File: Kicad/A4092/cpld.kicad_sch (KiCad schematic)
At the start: 15 parts, among them J2 Conn_01x06_Pin, U7 AMS1117-3.3, U9 XC95144XL-TQ144

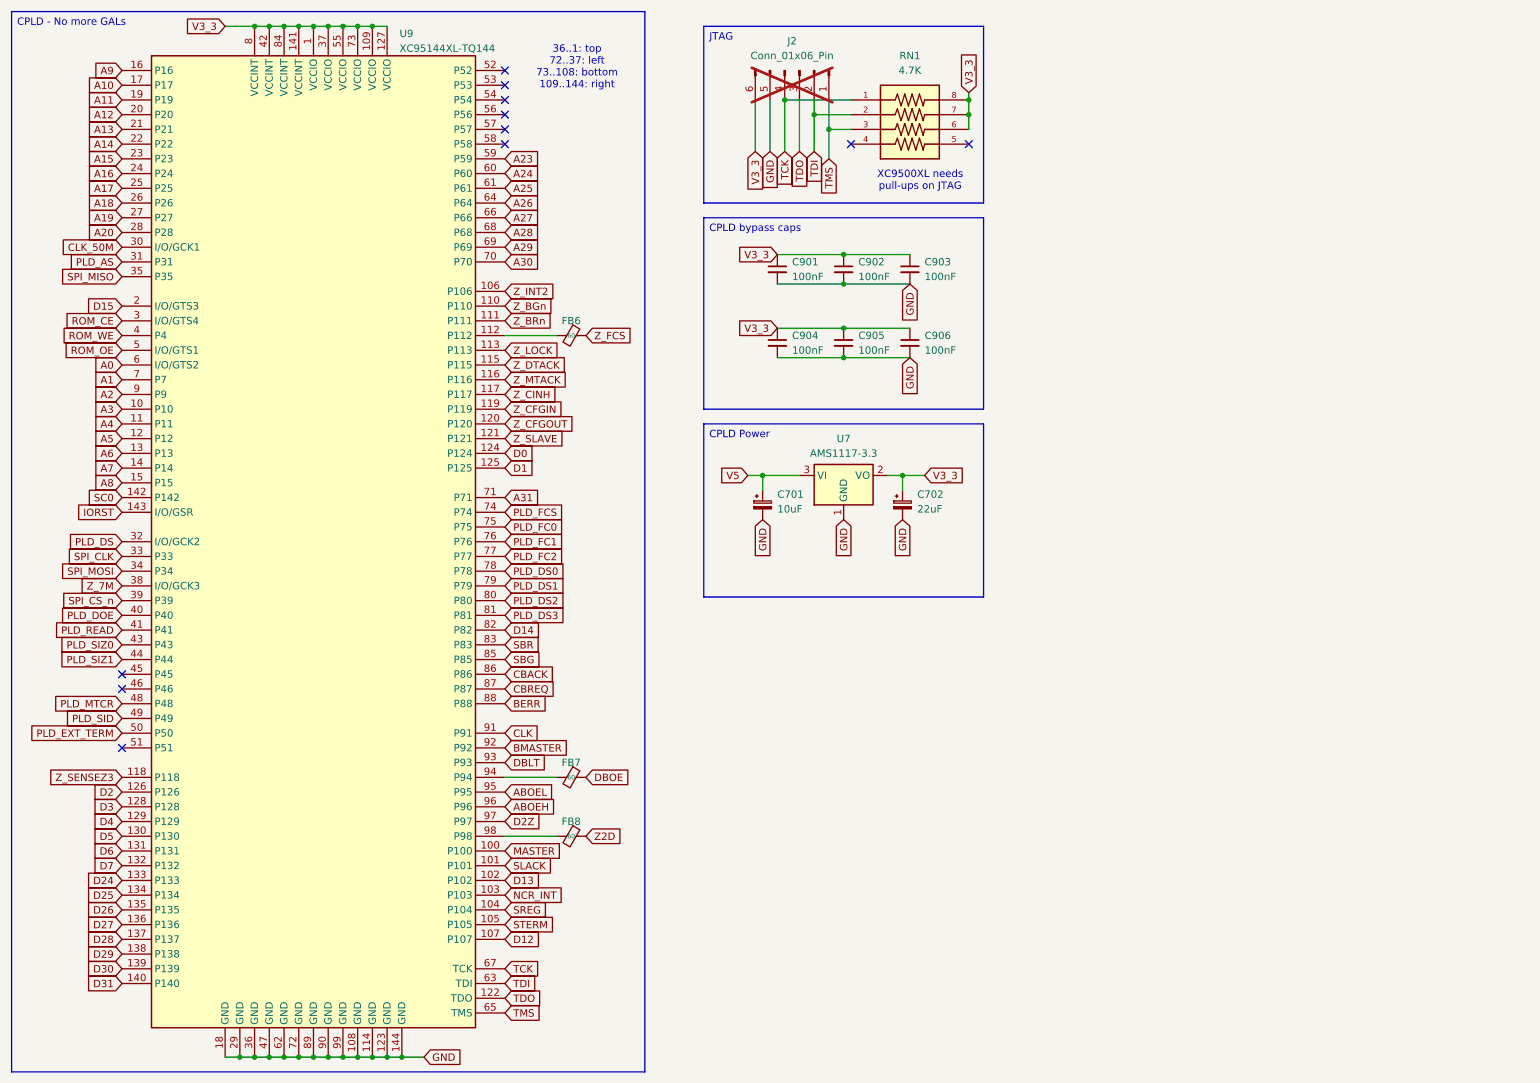
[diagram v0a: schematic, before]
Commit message: First version of A4770 cheetah
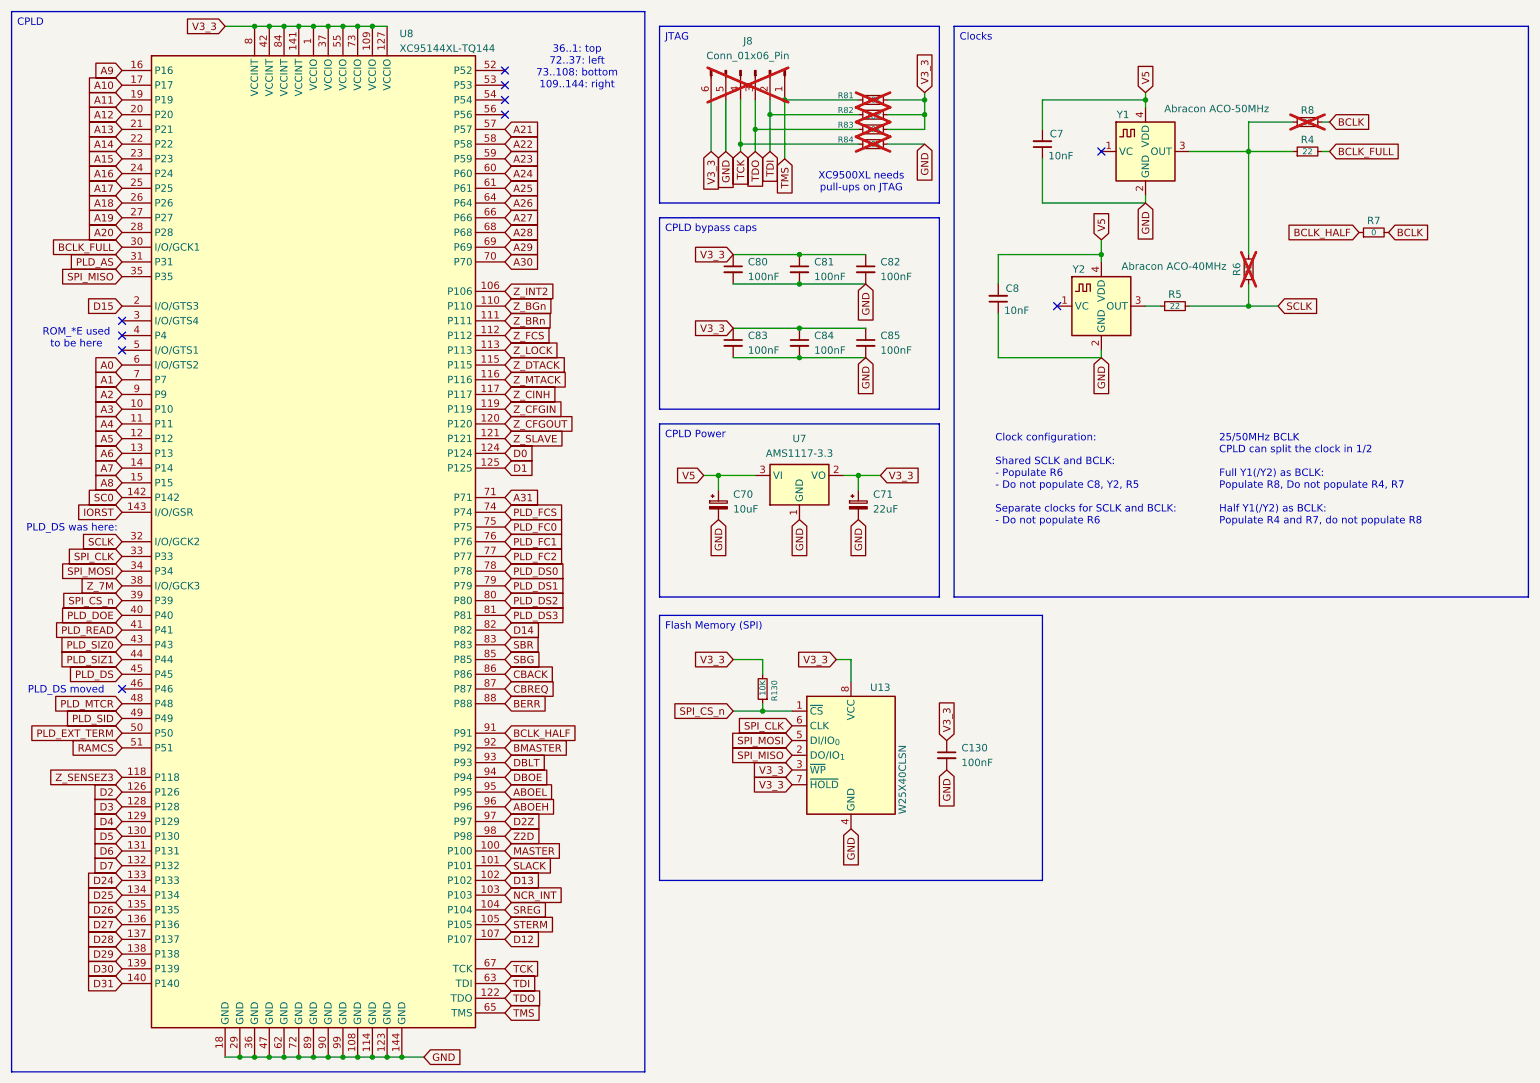
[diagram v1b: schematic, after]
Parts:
- removed FB6, FB7, FB8: 60, Capacitor_SMD:C_0603_1608Metric_Pad1.08x0.95mm_HandSolder, symbol Device:FerriteBead_Small
- removed RN1: 4.7K, CAY16_102J4LF:BO_CAY16, symbol YC324-FK-071KL:YC324-FK-071KL
- added C130: 100nF, Capacitor_SMD:C_0603_1608Metric_Pad1.08x0.95mm_HandSolder, symbol Device:C_Small
- added C7, C8: 10nF, Capacitor_SMD:C_0603_1608Metric_Pad1.08x0.95mm_HandSolder, symbol Device:C_Small
- added R130, R81, R82, R83, R84: 10K, Resistor_SMD:R_0603_1608Metric_Pad0.98x0.95mm_HandSolder, symbol Device:R_Small
- added R4, R5, R6, R8: 22, Resistor_SMD:R_0603_1608Metric, symbol Device:R_Small
- added R7: 0, Resistor_SMD:R_0603_1608Metric, symbol Device:R_Small
- added U13: W25X40CLSN, SOIC-8_multi:SOIC-8_multi, symbol Memory_Flash:W25X40CLSN
- added Y1: Abracon ACO-50MHz, Oscillator:Oscillator_SMD_Fox_FT5H_5.0x3.2mm, symbol Oscillator:FT5HV
- added Y2: Abracon ACO-40MHz, Oscillator:Oscillator_SMD_Fox_FT5H_5.0x3.2mm, symbol Oscillator:FT5HV
- renumbered C701 to C70, C702 to C71, C901 to C80, C902 to C81, C903 to C82, C904 to C83, C905 to C84, C906 to C85, J2 to J8, U9 to U8
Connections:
- net DBOE: now also U8.94 (P94)
- net GND: now also C130.2, C7.1, C8.1, R84.1, U13.4 (GND), Y1.2 (GND), Y2.2 (GND)
- net PLD_DS: now also U8.45 (P45); no longer U8.32 (I/O/GCK2)
- net SPI_CLK: now also U13.6 (CLK)
- net SPI_CS_n: now also R130.1, U13.1 (~{CS})
- net SPI_MISO: now also U13.2 (DO/IO_{1})
- net SPI_MOSI: now also U13.5 (DI/IO_{0})
- net TCK: now also R84.2
- net TDI: now also R82.2
- net TDO: now also R83.2
- net TMS: now also R81.2
- net V3_3: now also C130.1, R130.2, R81.1, R82.1, R83.1, U13.3 (~{WP}), U13.7 (~{HOLD}), U13.8 (VCC)
- net V5: now also C7.2, C8.2, Y1.4 (VDD), Y2.4 (VDD)
- net Z2D: now also U8.98 (P98)
- net Z_FCS: now also U8.112 (P112)
- net RAMCS: now reaches U8.51 (P51)
- net A21: now reaches U8.57 (P57)
- net A22: now reaches U8.58 (P58)
- net CLK renamed BCLK_HALF
- net BCLK_HALF: now also R7.1
- net CLK_50M renamed BCLK_FULL
- net BCLK_FULL: now also R4.2
- net ROM_CE: no longer names the net of U8.3 (I/O/GTS4)
- net ROM_OE: no longer names the net of U8.5 (I/O/GTS1)
- net ROM_WE: no longer names the net of U8.4 (P4)
- new net: R4.1, R6.2, R8.1, Y1.3 (OUT)
- new net: R5.1, Y2.3 (OUT)
- new net BCLK: R7.2, R8.2
- new net SCLK: R5.2, R6.1, U8.32 (I/O/GCK2)
- no-connect marks 11 -> 10
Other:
- note added: "25/50MHz BCLK CPLD can split the clock in 1/2 Full Y1(/Y2) as BCLK: Populate R8, Do not populate R4, R7 Half Y1(/Y2) as BCLK: Populate R4 and R7, do not populate R8"
- note added: "Clock configuration: Shared SCLK and BCLK: - Populate R6 - Do not populate C8, Y2, R5 Separate clocks for SCLK and BCLK: - Do not populate R6"
- note added: "PLD_DS moved"
- note added: "PLD_DS was here:"
- note added: "ROM_*E used to be here"
- moved on the sheet: C70, C71, C80, C81, C82, C83, C84, C85, J8, U7
